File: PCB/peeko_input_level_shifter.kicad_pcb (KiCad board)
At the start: 2 copper layers, 18.3 x 43.2 mm, 21 parts, among them J1 Conn_02x15_Odd_Even, J2 Conn_02x15_Odd_Even, U1 TXU0104, U2 TXU0104, U3 TXU0104, U4 TXU0104, U5 TXU0104, U6 TXU0104

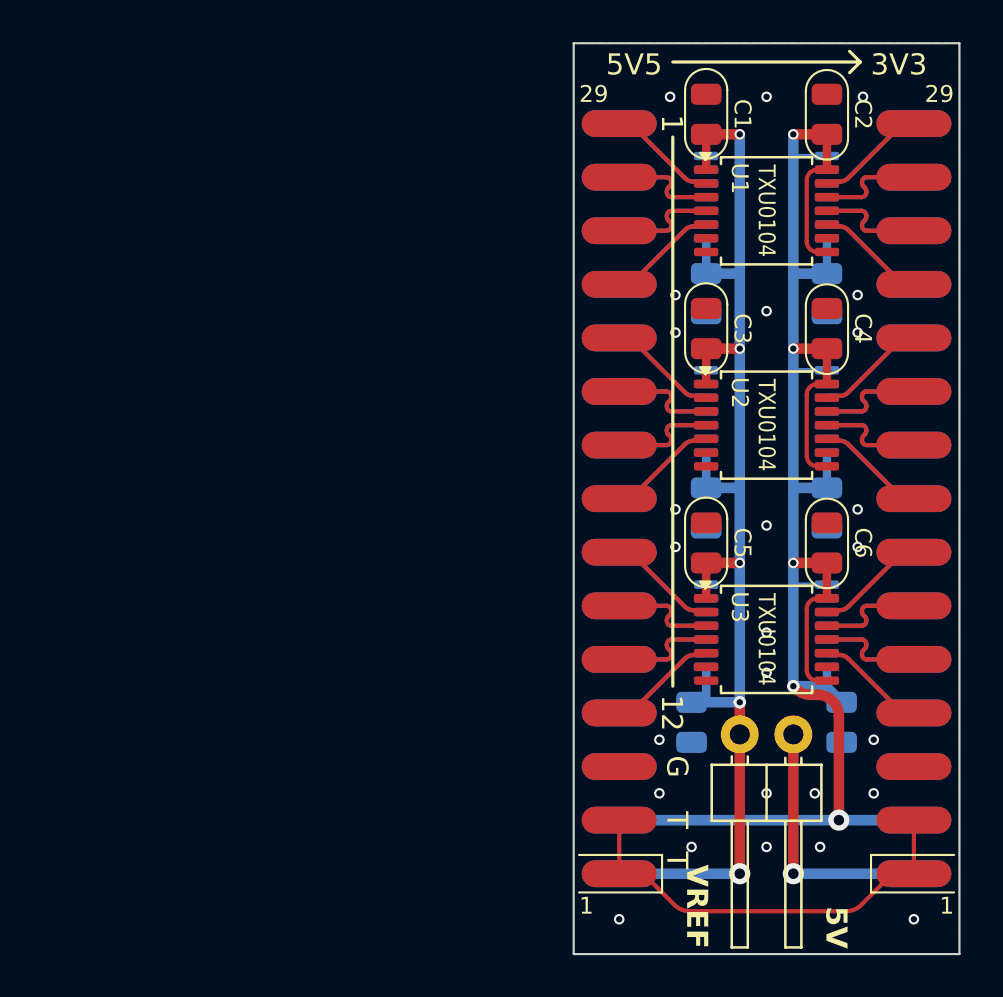
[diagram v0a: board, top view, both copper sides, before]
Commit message: pics
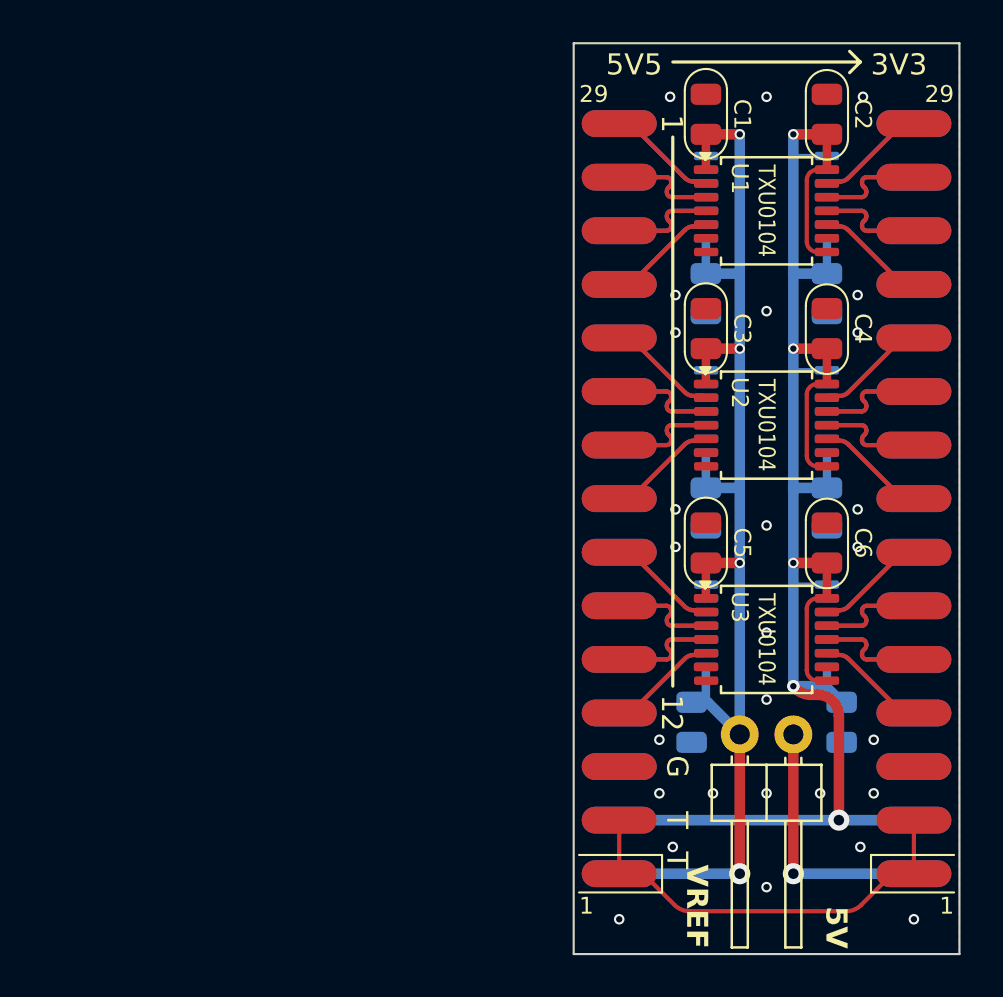
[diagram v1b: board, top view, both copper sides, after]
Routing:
- net VREF: track 60.4 -> 61.8 mm, vias 5 -> 4
- net +3V3: track 89.6 -> 88.6 mm
- net GND: vias 26 -> 27

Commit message: level shifter housing
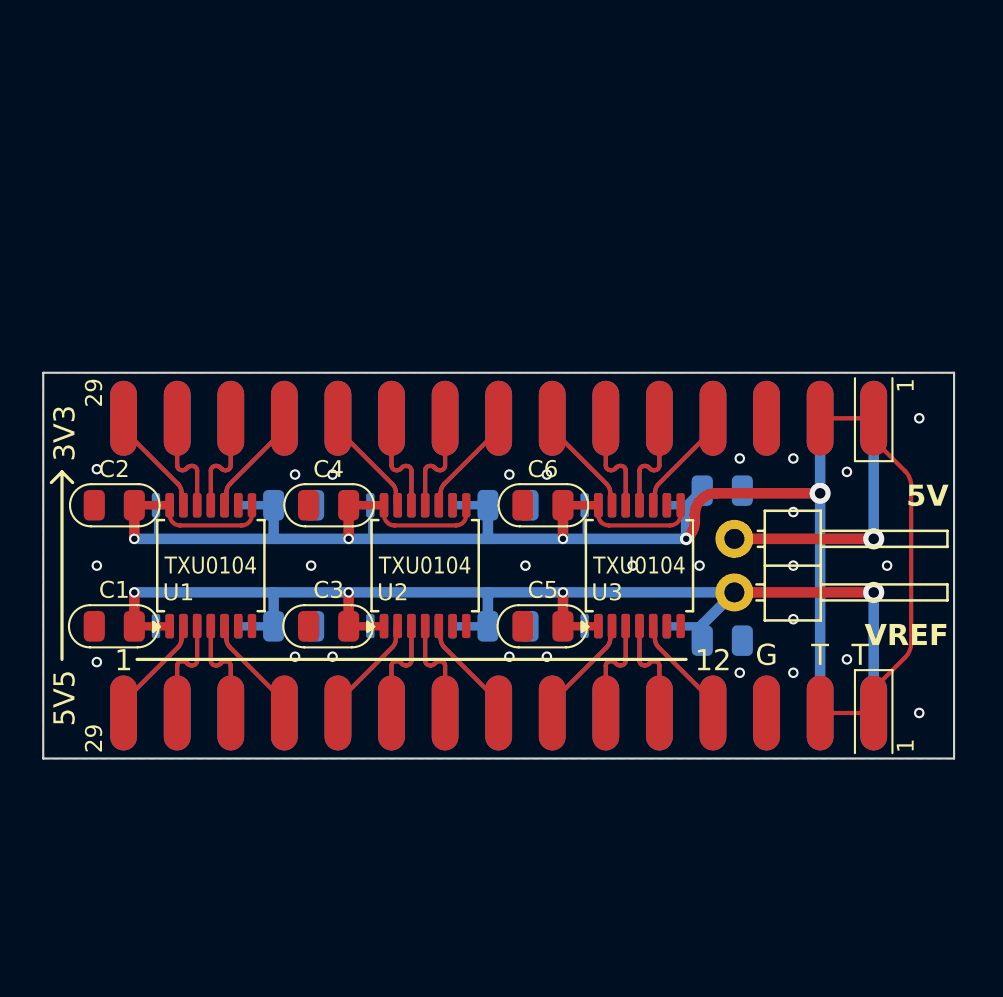
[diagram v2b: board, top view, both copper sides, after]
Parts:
- moved C2 38.5 mm to (129.0, 96.4), turned to 180 degrees
- moved C1 37.1 mm to (129.0, 102.1), turned to 0 degrees
- moved U6 32.2 mm to (132.9, 99.2), turned to 90 degrees
- moved U1 31.3 mm to (133.6, 99.2), turned to 90 degrees
- moved C12 27.2 mm to (137.5, 96.4), turned to 0 degrees
- moved C11 25.1 mm to (137.5, 102.1), turned to 180 degrees
- moved C4 25.1 mm to (139.1, 96.4), turned to 180 degrees
- moved C3 22.8 mm to (139.1, 102.1), turned to 0 degrees
- moved J2 22.6 mm to (147.2, 90.1), turned to -90 degrees
- moved U5 18.4 mm to (143.1, 99.2), turned to 90 degrees
- moved U2 17.5 mm to (143.7, 99.2), turned to 90 degrees
- moved C10 15.1 mm to (147.6, 96.4), turned to 0 degrees
- moved C6 13.6 mm to (149.3, 96.4), turned to 180 degrees
- moved J1 12.8 mm to (147.2, 108.4), turned to -90 degrees
- moved C8 12.4 mm to (157.8, 95.7), turned to 0 degrees
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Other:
- board size 18.3 x 43.2 mm -> 43.2 x 18.3 mm
